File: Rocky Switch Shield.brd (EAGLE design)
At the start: 68.4 x 47 mm, 14 parts

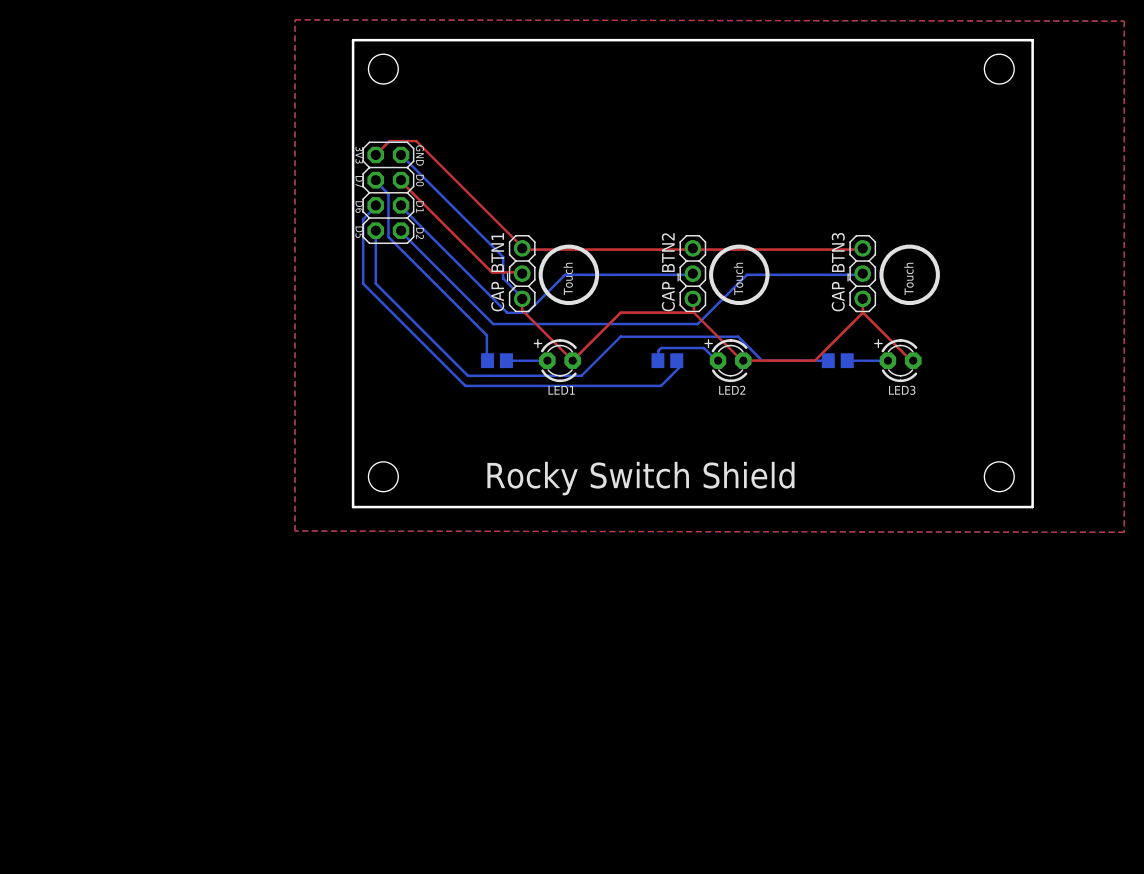
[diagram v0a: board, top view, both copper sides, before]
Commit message: Update new shield for rocky switch
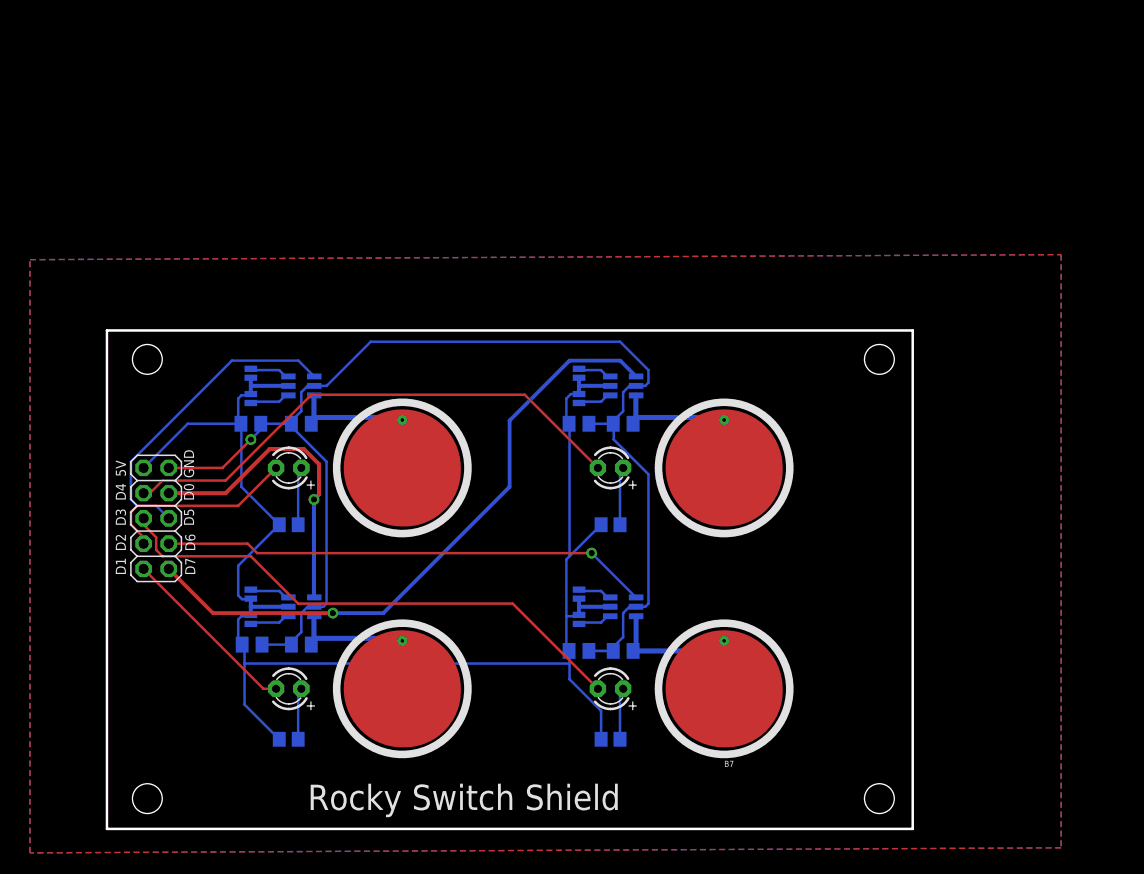
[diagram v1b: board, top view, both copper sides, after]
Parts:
- removed CAP_BTN1, CAP_BTN2, CAP_BTN3: (no value), adafruit:1X03
- removed JP2: (no value), adafruit:2X04
- added B5, B6, B7, B8: (no value), PatternAgents-TouchWidgets:BUTTON_PASSIVE_12MM
- added C1, C3, C5, C7: 30pF, rcl:C0805K
- added C2, C4, C6, C8: 0.1uF, rcl:C0805K
- added JP1: (no value), pinhead:2X05
- added LED4: (no value), adafruit:LED3MM
- added R4: 1K, rcl:R0805
- added SJ1, SJ2, SJ3, SJ4, SJ5, SJ6, SJ7, SJ8: JUMPER-PAD-2-NOYES_SILK, SparkFun-Passives:PAD-JUMPER-2-NO_YES_SILK
- added U$1, U$2, U$3, U$4: TTP223B, My Eagle Lib:SOT23-6
- moved LED2 45.8 mm to (18.4, 36.2), turned to 180 degrees
- moved R3 44.4 mm to (50.8, 8.89)
- moved LED3 44.1 mm to (50.8, 14.0), turned to 180 degrees
- moved R1 43.5 mm to (18.4, 8.89)
- moved LED1 42.8 mm to (18.4, 14.0), turned to 180 degrees
- moved R2 41.5 mm to (18.4, 30.5), turned to 180 degrees
- moved U$6 40.2 mm to (4.19, 2.92)
- moved U$9 37.6 mm to (4.19, 47.1)
- moved U$7 34.6 mm to (77.9, 2.92)
- moved U$8 31.6 mm to (77.9, 47.1)
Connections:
- removed net 3V3: CAP_BTN1.3, CAP_BTN2.3, CAP_BTN3.3, JP2.1
- new net D3: JP1.6, LED3.K
- new net D4: JP1.8, LED4.K
- new net I1: B5.BUTTON, C1.1, U$1.3
- new net I2: B6.BUTTON, C3.1, U$2.3
- new net I3: B7.BUTTON, C5.1, U$3.3
- new net I4: B8.BUTTON, C7.1, U$4.3
- new net N$1: SJ1.1, U$1.4
- new net N$11: SJ5.1, U$3.4
- new net N$12: SJ6.1, U$3.6
- new net N$15: SJ7.1, U$4.4
- new net N$16: SJ8.1, U$4.6
- new net N$5: SJ2.1, U$1.6
- new net N$7: SJ3.1, U$2.4
- new net N$8: SJ4.1, U$2.6
- new net N$9: LED4.A, R4.2
- new net VDD: C2.1, C4.1, C6.1, C8.1, JP1.10, R1.1, R2.1, R3.1, R4.1, SJ1.2, SJ2.2, SJ3.2, SJ4.2, SJ5.2, SJ6.2, SJ7.2, SJ8.2, U$1.5, U$2.5, U$3.5, U$4.5
- net D0: now also JP1.7, U$1.1; no longer CAP_BTN1.2, JP2.4
- net D1: now also JP1.2, LED1.K; no longer CAP_BTN2.2, JP2.6
- net D2: now also JP1.4, LED2.K; no longer CAP_BTN3.2, JP2.8
- net D5: now also JP1.5, U$2.1; no longer JP2.7, R3.1
- net D6: now also JP1.3, U$3.1; no longer JP2.5, R2.1
- net D7: now also JP1.1, U$4.1; no longer JP2.3, R1.1
- net GND: now also C1.2, C2.2, C3.2, C4.2, C5.2, C6.2, C7.2, C8.2, JP1.9, U$1.2, U$2.2, U$3.2, U$4.2; no longer CAP_BTN1.1, CAP_BTN2.1, CAP_BTN3.1, JP2.2, LED1.K, LED2.K, LED3.K
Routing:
- net VDD: track 0.00 -> 150.5 mm
- net 3V3: track 54.4 -> 0.00 mm
- net D3: track 0.00 -> 53.9 mm
- net D4: track 0.00 -> 52.9 mm
- net GND: track 72.9 -> 125.8 mm, vias 0 -> 1
- net D7: track 22.9 -> 64.0 mm, vias 0 -> 1
- net D2: track 52.5 -> 20.1 mm
- net D5: track 57.3 -> 31.8 mm
- net D1: track 35.5 -> 18.3 mm
- net D0: track 16.2 -> 31.2 mm, vias 0 -> 1
- net I3: track 0.00 -> 13.2 mm
- net I1: track 0.00 -> 13.0 mm
- net I2: track 0.00 -> 13.0 mm
- net I4: track 0.00 -> 13.0 mm
- net N$9: track 0.00 -> 5.85 mm
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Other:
- board size 68.4 x 47 mm -> 81.1 x 50.2 mm
- board text added: "5V"
- board text added: "D3"
- board text added: "D4"
- board text removed: "3V3"
- board text removed: "Touch"

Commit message: Update board design to version 0.2
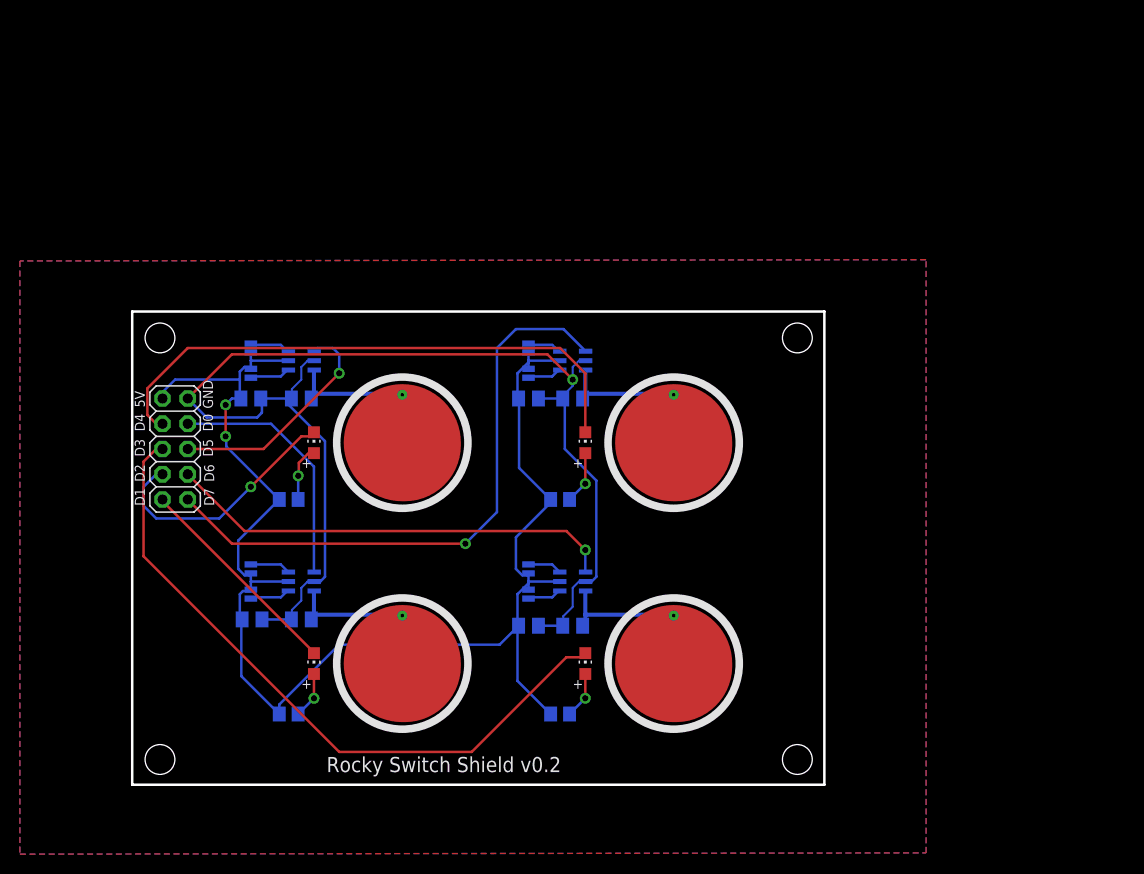
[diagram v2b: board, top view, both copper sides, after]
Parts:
- LED1, LED2, LED3, LED4: device adafruit:LED3MM -> adafruit:CHIP-LED0805
- SJ1, SJ3, SJ5, SJ7: value JUMPER-PAD-2-NOYES_SILK -> AHLB
- SJ2, SJ4, SJ6, SJ8: value JUMPER-PAD-2-NOYES_SILK -> TOG
- moved U$7 9.15 mm to (69.6, 6.86)
- moved U$8 8.53 mm to (69.6, 49.3)
- moved JP1 7.24 mm to (6.99, 38.1)
- moved B7 5.68 mm to (57.1, 16.5)
- moved R4 5.68 mm to (45.7, 33.0)
- moved SJ5 5.68 mm to (42.5, 23.5)
- moved B8 5.68 mm to (57.1, 38.7)
- moved C5 5.68 mm to (47.0, 20.3)
- moved C6 5.68 mm to (42.5, 20.3)
- moved C7 5.68 mm to (47.0, 43.2)
- moved C8 5.68 mm to (42.5, 43.2)
- moved R3 5.68 mm to (45.7, 11.4)
- moved SJ6 5.68 mm to (42.5, 26.0)
- moved SJ7 5.68 mm to (42.5, 45.7)
- moved SJ8 5.68 mm to (42.5, 48.3)
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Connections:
- net D1: now also LED1.C; no longer LED1.K
- net D2: now also LED2.C; no longer LED2.K
- net D3: now also LED3.C; no longer LED3.K
- net D4: now also LED4.C; no longer LED4.K
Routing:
- net D3: track 53.9 -> 68.7 mm
- net D5: track 31.8 -> 23.2 mm, vias 0 -> 1
- net VDD: track 150.5 -> 142.5 mm, vias 0 -> 2
- net D0: track 31.2 -> 25.1 mm, vias 1 -> 0
- net D2: track 20.1 -> 25.6 mm, vias 0 -> 1
- net D4: track 52.9 -> 57.4 mm
- net D6: track 49.3 -> 45.4 mm
- net D1: track 18.3 -> 21.8 mm
- net D7: track 64.0 -> 61.4 mm
- net N$9: track 5.85 -> 5.33 mm, vias 0 -> 1
- net N$6: track 5.21 -> 4.69 mm, vias 0 -> 1
- net N$3: track 5.21 -> 4.69 mm, vias 0 -> 1
- net I3: track 13.2 -> 12.7 mm
- net N$4: track 5.85 -> 5.68 mm, vias 0 -> 1
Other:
- board size 81.1 x 50.2 mm -> 69.6 x 47.6 mm
- board text added: "Rocky Switch Shield v0.2"
- board text removed: "Rocky Switch Shield"
